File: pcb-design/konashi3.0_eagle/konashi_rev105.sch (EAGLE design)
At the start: 35 parts, among them CN1 ZX62-B-5PA(11), CN2 S2B-PH-K-S, CN3 WML-C69, CN4 2X07, CN7 BK-913, IC1 LP2985N, IC2 ZLDO1117G50DITR-ND

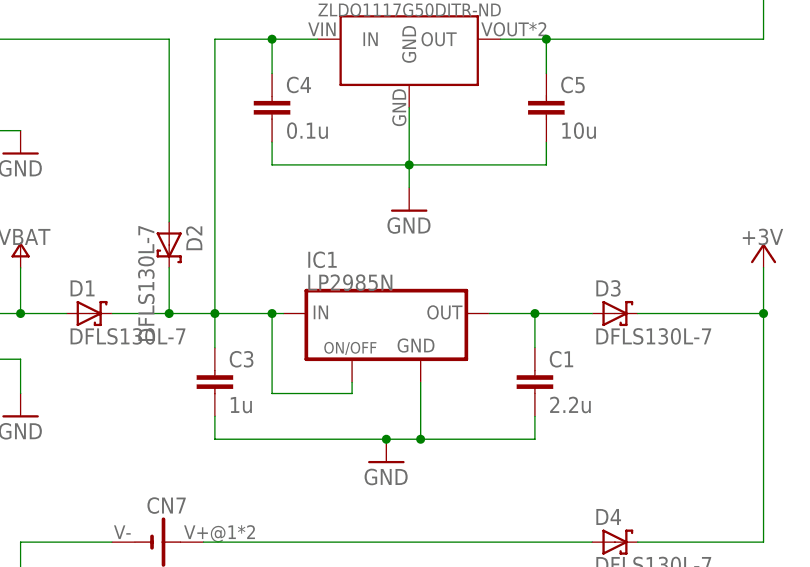
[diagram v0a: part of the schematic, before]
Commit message: BOM追加
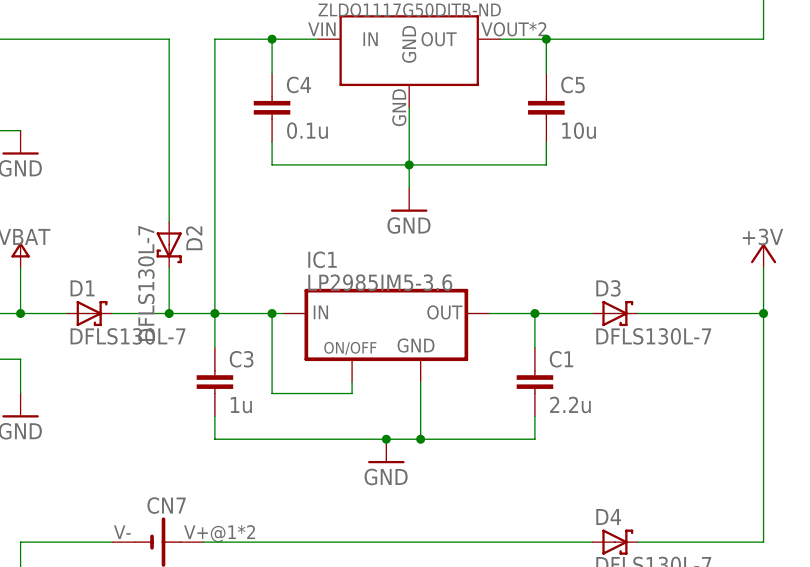
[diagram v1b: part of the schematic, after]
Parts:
- IC1: value LP2985N -> LP2985IM5-3.6
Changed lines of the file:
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@@
 <part name="R2" library="rcl" deviceset="R-EU_" device="R0603" value="3.3k"/>
 <part name="U$10" library="supply" deviceset="+3V" device=""/>
-<part name="IC1" library="LDO" deviceset="LP2981-30DBVR" device="" value="LP2985N"/>
+<part name="IC1" library="LDO" deviceset="LP2981-30DBVR" device="" value="LP2985IM5-3.6"/>
 <part name="CN7" library="con-CoinBatt" deviceset="BK-913" device=""/>
 <part name="SJ2" library="pad" deviceset="SJS" device=""/>
